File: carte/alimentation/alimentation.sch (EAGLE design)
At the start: 1 part

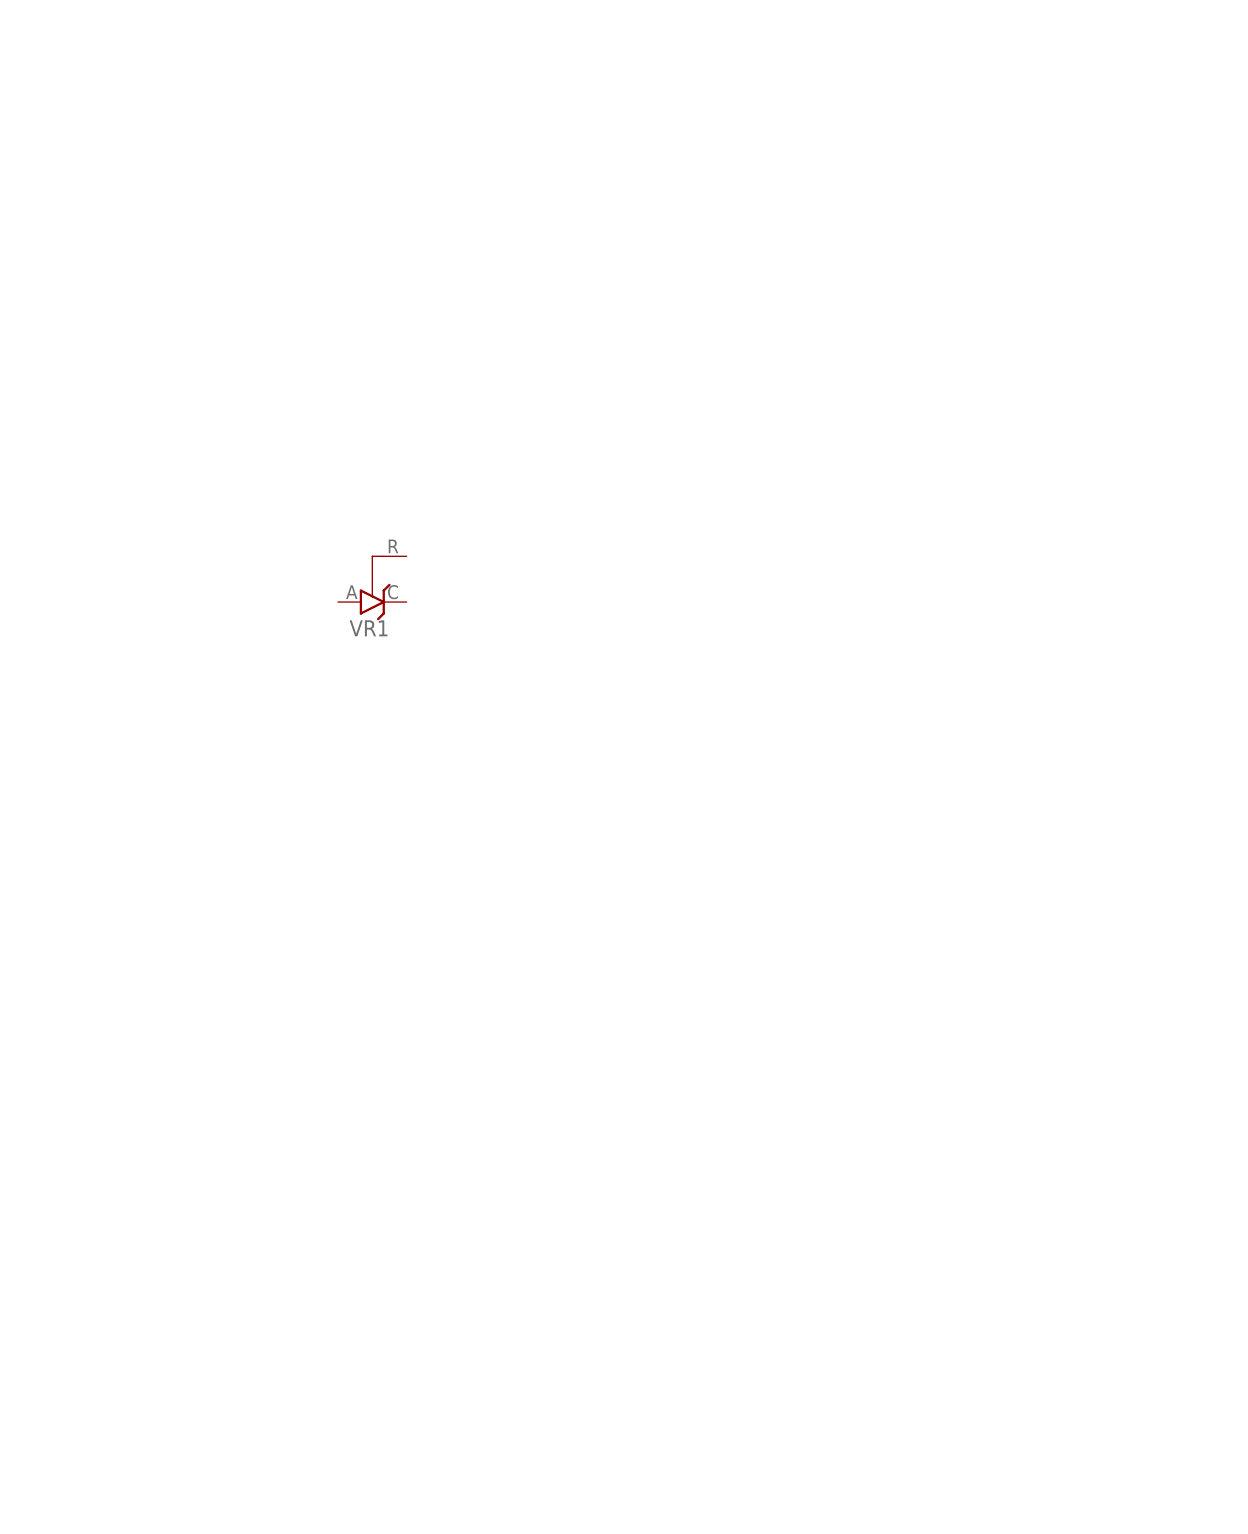
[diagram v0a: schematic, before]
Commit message: MAJ layout carte alim
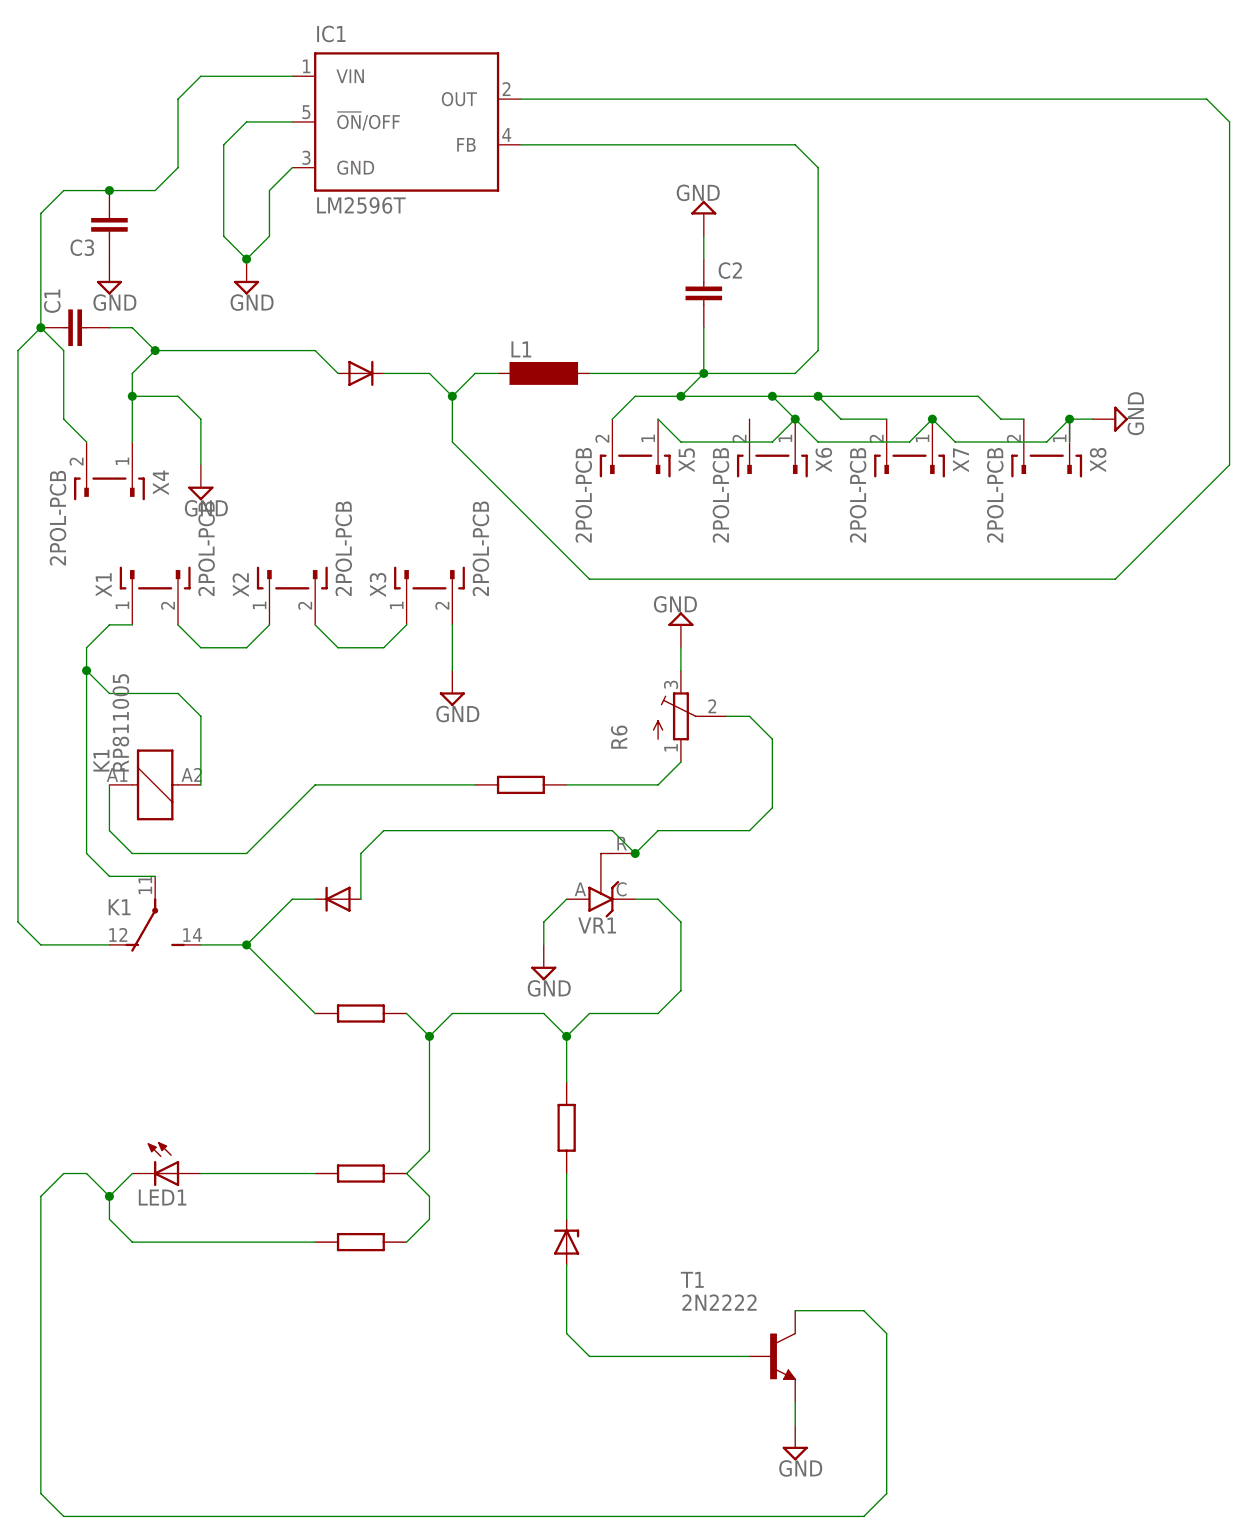
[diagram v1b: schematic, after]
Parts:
- added C1, C2, C3: (no value), capacitor-wima:C5/3.5
- added IC1: LM2596T, national-semiconductor:LM2596T
- added K1: RP811005, relay:RP811005
- added L1: (no value), inductor-neosid:SM-L15A
- added LED1: (no value), eagle-ltspice:LED_E
- added R6: (no value), pot:TRIM_EU-3223G
- added T1: 2N2222, transistor:2N2222
- added X1, X2, X3, X4, X5, X6, X7, X8: 2POL-PCB, con-friwo:2POL-PCB
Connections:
- new net GND: C1.2, C2.1, C2.2, C3.1, IC1.!ON!/OFF, IC1.FB, IC1.GND, L1.2, R6.E, T1.E, VR1.A, X3.2, X4.1, X5.1, X5.2, X6.1, X7.1, X7.2, X8.1, X8.2
- new net N$10: VR1.C
- new net N$12: T1.B
- new net N$13: LED1.C, T1.C
- new net N$14: LED1.A
- new net N$16: IC1.OUT, L1.1
- new net N$17: C1.1, C3.2, IC1.VIN, K12.O, X4.2
- new net N$3: K11.2, K12.P, X1.1
- new net N$4: X1.2, X2.1
- new net N$5: X2.2, X3.1
- new net N$6: K11.1
- new net N$7: K12.S
- new net N$8: R6.S, VR1.R
- new net N$9: R6.A
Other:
- moved on the sheet: VR1
